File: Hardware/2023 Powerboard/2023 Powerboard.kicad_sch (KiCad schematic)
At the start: 155 parts, among them J1 RJ45_LED_Shielded, J2 6P6C, Q1 BSS138, Q10 BSS138, Q11 QM6015D, Q12 IRF7606PBF, Q13 BSS138, Q14 QM6015D, Q15 BSS138, Q16 IRF7606PBF, Q17 BSS138, Q18 QM6015D, Q19 BSS138, Q2 BSS138, Q20 BSS138, Q21 IRF7606PBF, Q22 QM6015D, Q23 BSS138, Q24 BSS138, Q25 IRF7606PBF, Q26 QM6015D, Q27 BSS138, Q28 BSS138, Q29 IRF7606PBF, Q3 QM6015D, Q30 QM6015D, Q31 BSS138, Q32 QM6015D, Q4 IRF7606PBF, Q5 BSS138, Q6 BSS138, Q7 QM6015D, Q8 IRF7606PBF, Q9 BSS138, U1 3V3, U2 Teensy4.1_DEV-16771

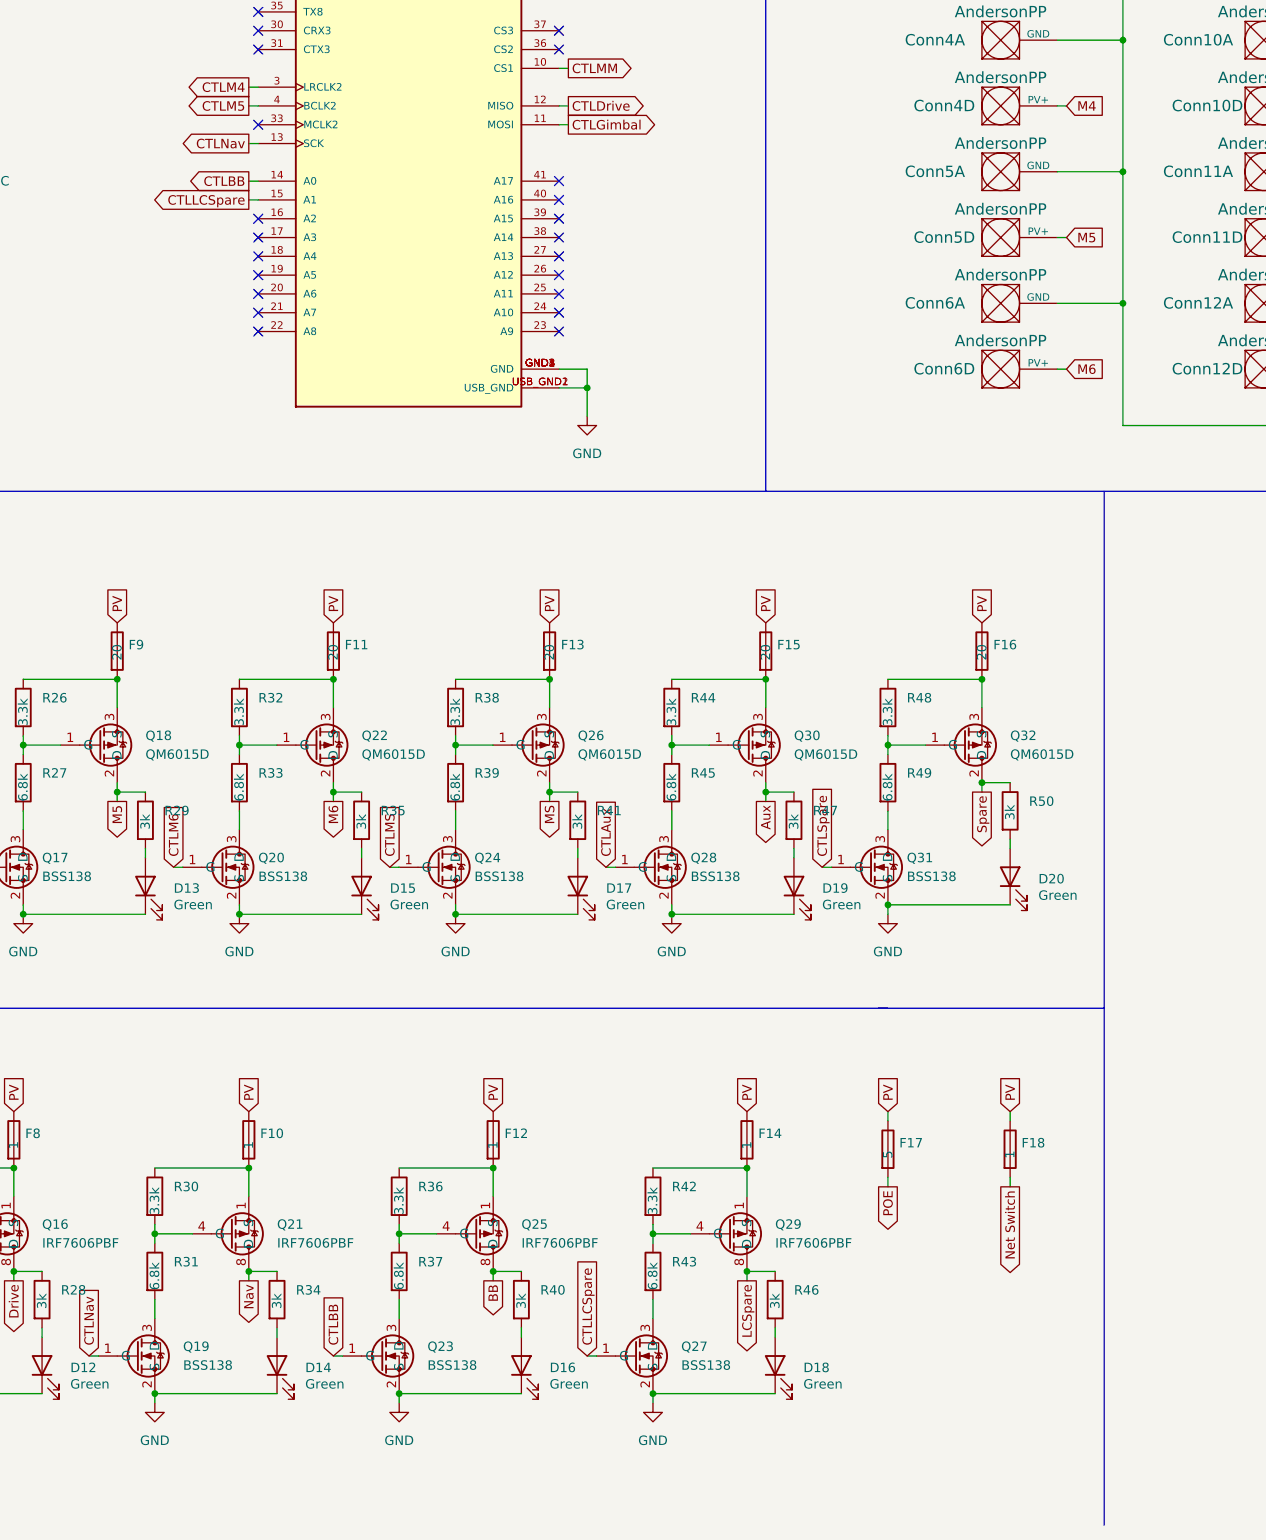
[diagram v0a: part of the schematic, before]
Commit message: Layout Review Changes
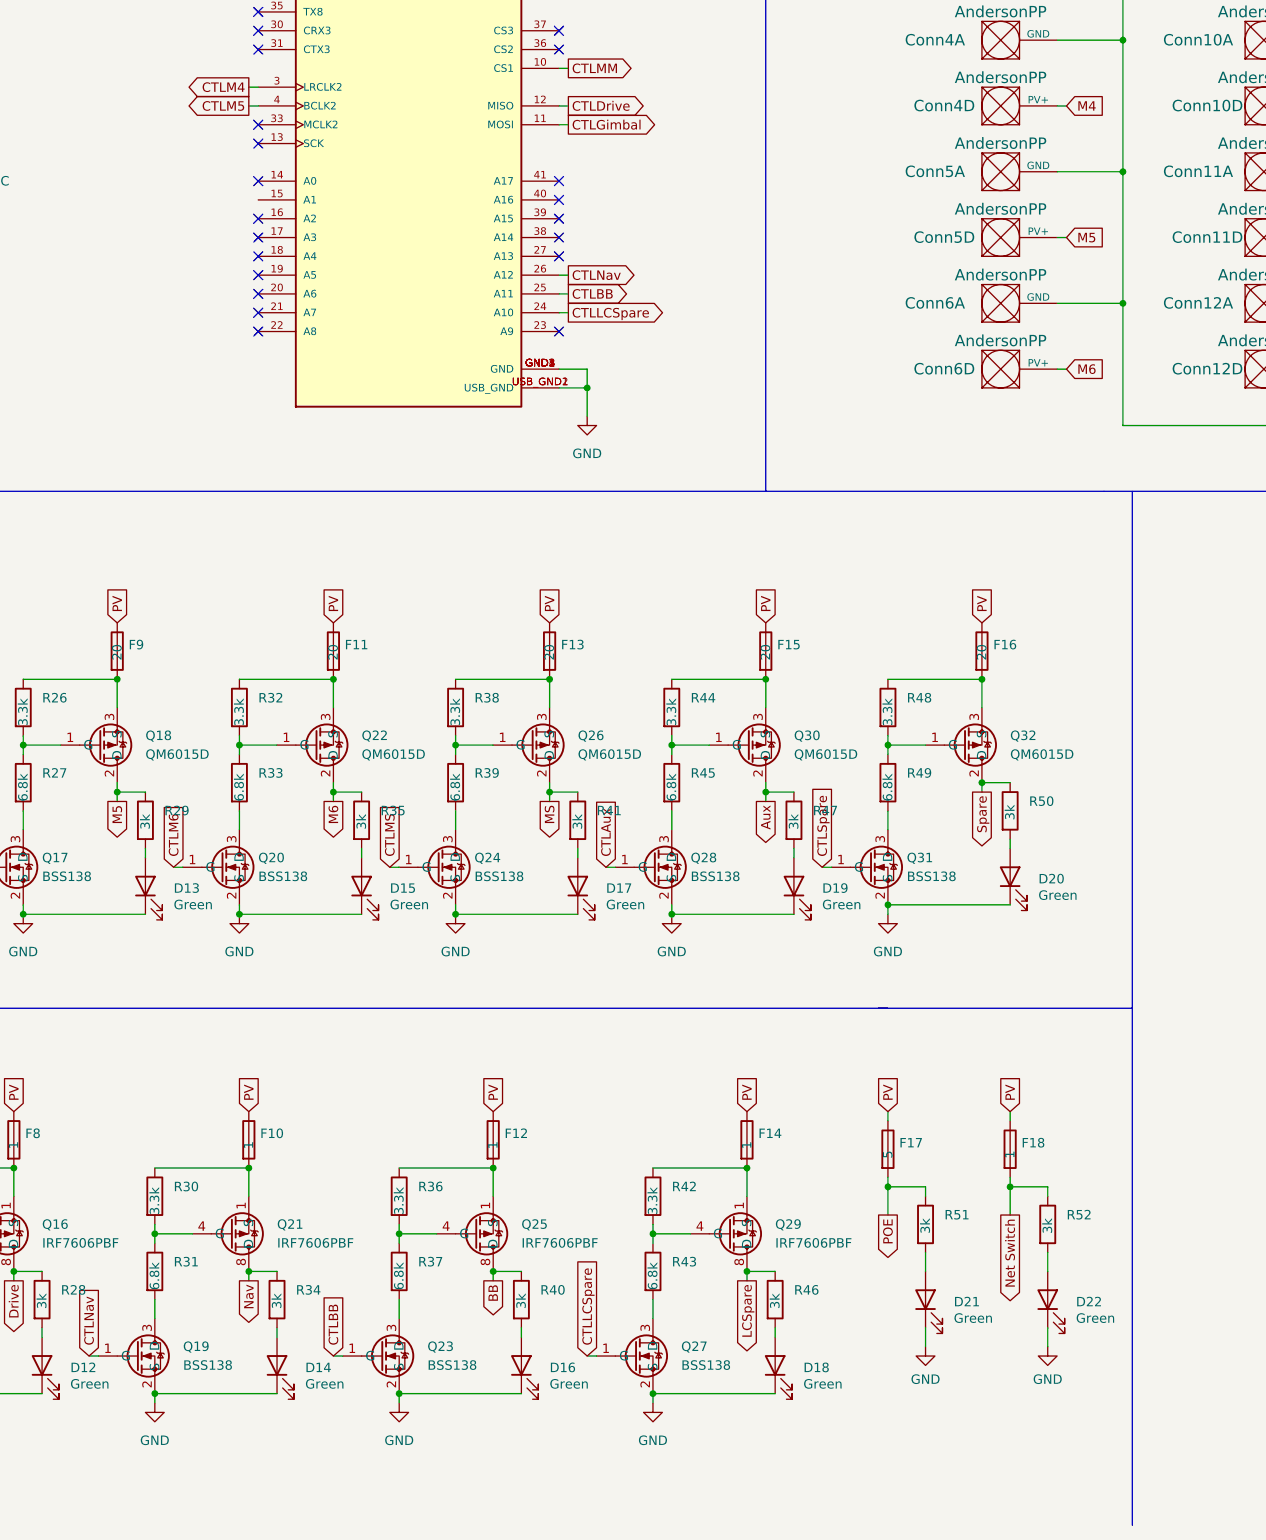
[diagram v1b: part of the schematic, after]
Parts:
- added D21, D22: Green, LED_SMD:LED_0603_1608Metric_Pad1.05x0.95mm_HandSolder, symbol Device:LED
- added R51, R52: 3k, Resistor_SMD:R_0603_1608Metric_Pad0.98x0.95mm_HandSolder, symbol Device:R
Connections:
- net CTLBB: now also U2.25 (A11); no longer U2.14 (A0)
- net CTLLCSpare: now also U2.24 (A10); no longer U2.15 (A1)
- net CTLNav: now also U2.26 (A12); no longer U2.13 (SCK)
- net GND: now also D21.1 (K), D22.1 (K)
- net Net Switch: now also R52.1
- net POE: now also R51.1
- new net: D21.2 (A), R51.2
- new net: D22.2 (A), R52.2
- no-connect marks 42 -> 41
